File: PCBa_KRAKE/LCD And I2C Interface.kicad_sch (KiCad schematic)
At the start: 44 parts, among them Q301 BSS138, Q401 BSS138, Q402 BSS138, U301 PCF8574AT_3_518, U302 LCD_20x4_Character-GPAD_SCH_L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, U303 Conn_01x16

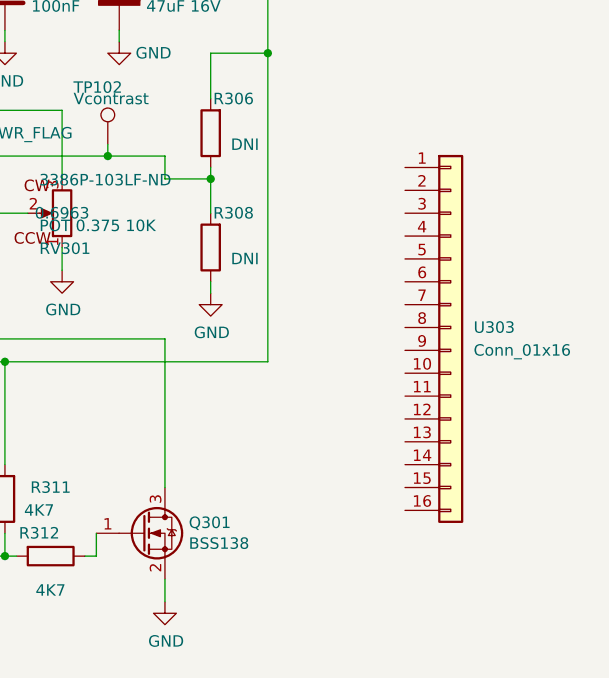
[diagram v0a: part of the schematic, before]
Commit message: USB_UART.kicad_sch, flipped the emmiter and the collctor for Q207. Added NC symbols for U303.
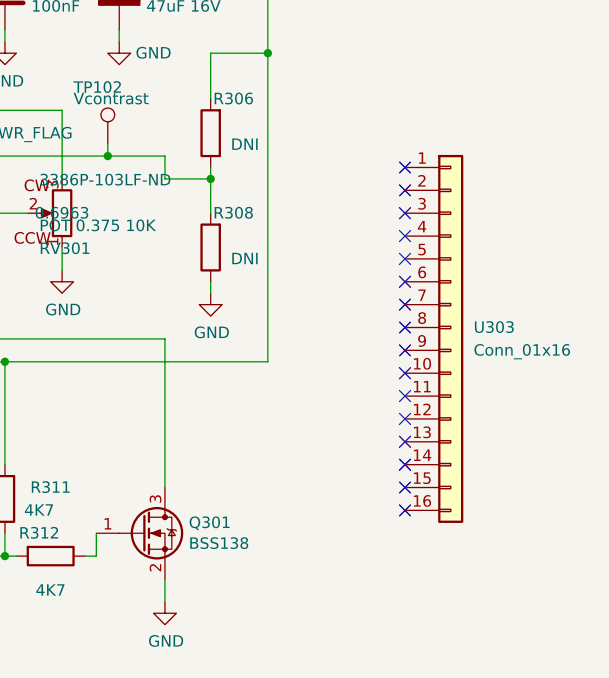
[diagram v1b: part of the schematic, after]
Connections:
- no-connect marks 0 -> 16
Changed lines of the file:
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@@
   (junction (at 167.64 52.07) (diameter 0) (color 0 0 0 0)
   )
+  (no_connect (at 247.65 81.28))
+  (no_connect (at 247.65 86.36))
+  (no_connect (at 247.65 91.44))
+  (no_connect (at 247.65 68.58))
+  (no_connect (at 247.65 76.2))
+  (no_connect (at 247.65 73.66))
+  (no_connect (at 247.65 63.5))
+  (no_connect (at 247.65 93.98))
+  (no_connect (at 247.65 88.9))
+  (no_connect (at 247.65 99.06))
+  (no_connect (at 247.65 101.6))
+  (no_connect (at 247.65 66.04))
+  (no_connect (at 247.65 71.12))
+  (no_connect (at 247.65 78.74))
+  (no_connect (at 247.65 96.52))
+  (no_connect (at 247.65 83.82))
   (wire (pts (xy 175.26 77.47) (xy 173.99 77.47))
     (stroke (width 0) (type default))
@@
   )
   (symbol (lib_id "Connector_Generic:Conn_01x16") (at 252.73 81.28 0) (unit 1)
-    (in_bom yes) (on_board yes) (dnp no) (fields_autoplaced)
+    (in_bom yes) (on_board no) (dnp no) (fields_autoplaced)
     (property "Reference" "U303" (at 255.27 81.28 0)
       (effects (font (size 1.27 1.27)) (justify left))
